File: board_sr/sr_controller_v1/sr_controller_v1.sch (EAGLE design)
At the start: 120 parts, among them IC2 74HC595D, J2 WIRE_HOLE-14AWG, J3 WIRE_HOLE-14AWG, J4 WIRE_HOLE-14AWG, J5 WIRE_HOLE-14AWG, J6 WIRE_HOLE-14AWG, J7 WIRE_HOLE-14AWG, Q1 32kHz, Q3 IRF5210

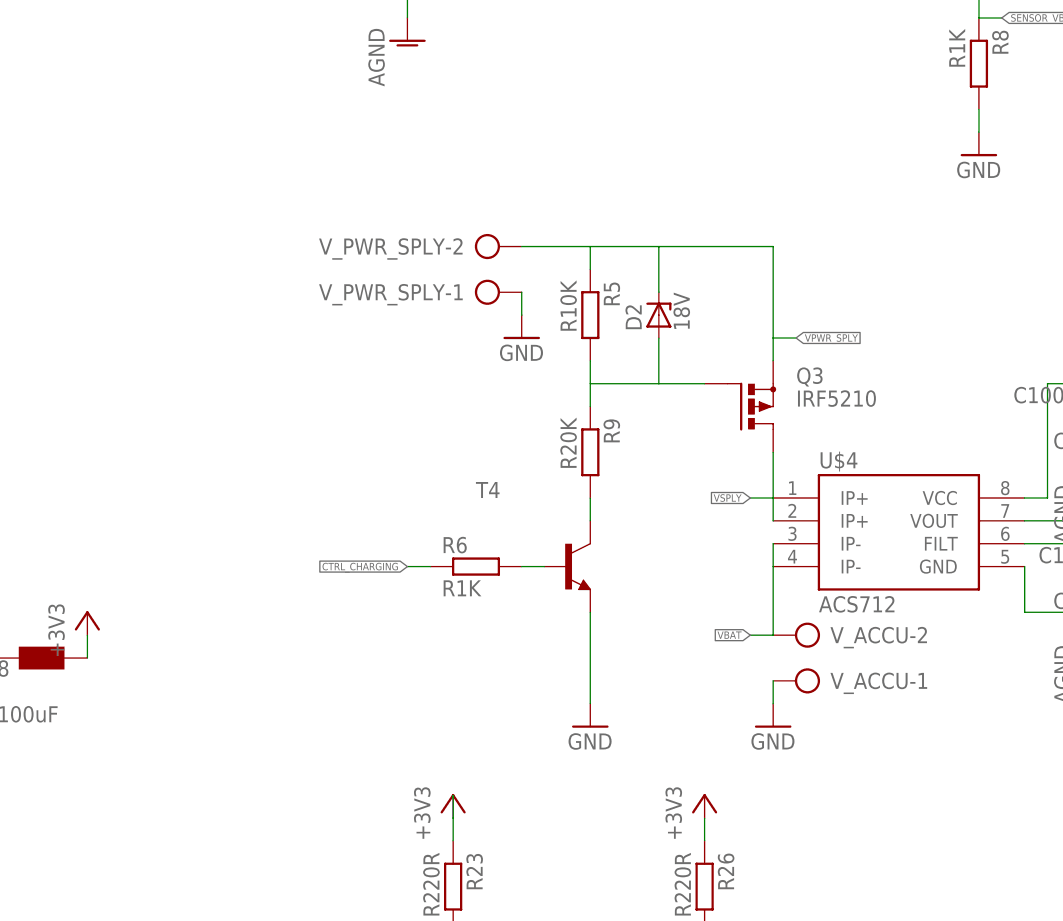
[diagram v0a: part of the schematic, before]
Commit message: Finish Routing PCB ver1 revA
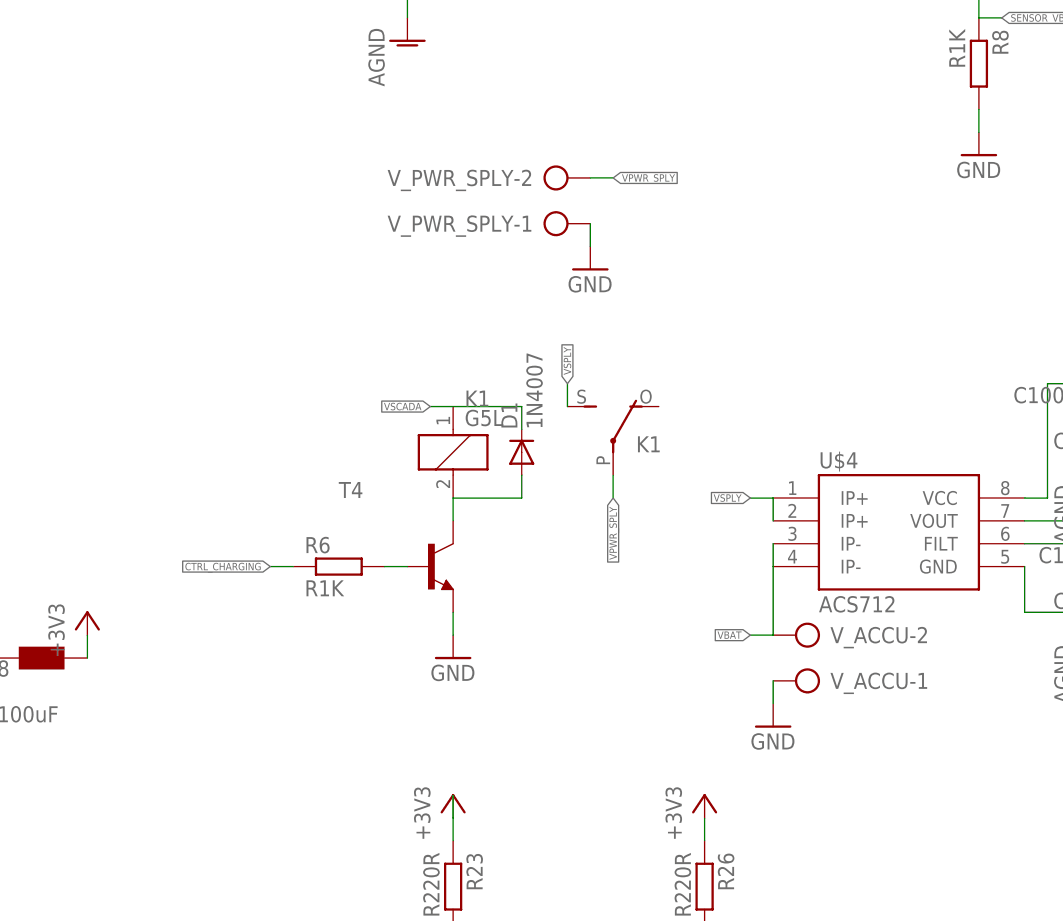
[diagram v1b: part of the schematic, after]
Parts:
- removed D2: 18V, diode:ZENER-DIODEDO41Z10
- removed Q3: IRF5210, transistor-power:PMOSFET_PTO220BV
- removed R5: R10K, resistor:R-EU_R0805
- removed R9: R20K, resistor:R-EU_R0805
- added D1: 1N4007, diode:DIODE-DO214AA
- added K1: G5L, relay:G5L
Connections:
- removed net N$11: D2.A, Q3.G, R5.2, R9.1
- removed net N$14: R9.2, T4.C
- new net N$34: D1.A, K11.2, T4.C
- net VPWR_SPLY: now also K12.P; no longer D2.C, Q3.S, R5.1
- net VSCADA: now also D1.C, K11.1
- net VSPLY: now also K12.S; no longer Q3.D
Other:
- moved on the sheet: R6, T4, V_PWR_SPLY-1, V_PWR_SPLY-2
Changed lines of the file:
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@@
 <part name="V_PWR_SPLY" library="con-ptr500" deviceset="AK300/2" device=""/>
 <part name="V_ACCU" library="con-ptr500" deviceset="AK300/2" device=""/>
-<part name="Q3" library="transistor-power" deviceset="PMOSFET_P" device="TO220BV" value="IRF5210"/>
 <part name="GND15" library="supply1" deviceset="GND" device=""/>
-<part name="R5" library="resistor" deviceset="R-EU_" device="R0805" value="R10K"/>
 <part name="GND16" library="supply1" deviceset="GND" device=""/>
 <part name="GND17" library="supply1" deviceset="GND" device=""/>
@@
 <part name="AGND3" library="supply1" deviceset="AGND" device=""/>
 <part name="GND19" library="supply1" deviceset="GND" device=""/>
-<part name="R9" library="resistor" deviceset="R-EU_" device="R0805" value="R20K"/>
-<part name="D2" library="diode" deviceset="ZENER-DIODE" device="DO41Z10" value="18V"/>
 <part name="U$4" library="SparkFun-AnalogIC" deviceset="ACS712" device=""/>
 <part name="C5" library="resistor" deviceset="C-EU" device="C0805K" value="C100N"/>
@@
 <part name="J6" library="powercube" deviceset="WIRE_HOLE-14AWG" device=""/>
 <part name="J7" library="powercube" deviceset="WIRE_HOLE-14AWG" device=""/>
+<part name="K1" library="relay" deviceset="G5L" device=""/>
+<part name="D1" library="diode" deviceset="DIODE-" device="DO214AA" value="1N4007"/>
 </parts>
 <sheets>
@@
 <instance part="VAC" gate="-1" x="177.8" y="231.14"/>
 <instance part="VAC" gate="-2" x="177.8" y="236.22"/>
-<instance part="V_PWR_SPLY" gate="-1" x="231.14" y="185.42"/>
-<instance part="V_PWR_SPLY" gate="-2" x="231.14" y="190.5"/>
+<instance part="V_PWR_SPLY" gate="-1" x="238.76" y="193.04"/>
+<instance part="V_PWR_SPLY" gate="-2" x="238.76" y="198.12"/>
 <instance part="V_ACCU" gate="-1" x="269.24" y="142.24" rot="R180"/>
 <instance part="V_ACCU" gate="-2" x="269.24" y="147.32" rot="R180"/>
-<instance part="Q3" gate="G$1" x="261.62" y="172.72"/>
 <instance part="GND15" gate="1" x="264.16" y="137.16"/>
-<instance part="R5" gate="G$1" x="243.84" y="182.88" rot="R270"/>
-<instance part="GND16" gate="1" x="236.22" y="180.34"/>
-<instance part="GND17" gate="1" x="243.84" y="137.16"/>
-<instance part="R6" gate="G$1" x="231.14" y="154.94"/>
+<instance part="GND16" gate="1" x="243.84" y="187.96"/>
+<instance part="GND17" gate="1" x="228.6" y="144.78"/>
+<instance part="R6" gate="G$1" x="215.9" y="154.94"/>
 <instance part="R7" gate="G$1" x="287.02" y="223.52" rot="R270"/>
 <instance part="R8" gate="G$1" x="287.02" y="210.82" rot="R270"/>
@@
 <instance part="AGND3" gate="VR1" x="320.04" y="213.36"/>
 <instance part="GND19" gate="1" x="309.88" y="213.36"/>
-<instance part="R9" gate="G$1" x="243.84" y="167.64" rot="R270"/>
-<instance part="D2" gate="G$1" x="251.46" y="182.88" rot="R90"/>
 <instance part="U$4" gate="G$1" x="279.4" y="157.48"/>
 <instance part="C5" gate="G$1" x="299.72" y="170.18" rot="R180"/>
@@
 <instance part="U$6" gate="G$1" x="48.26" y="78.74"/>
 <instance part="U$7" gate="G$1" x="48.26" y="45.72"/>
-<instance part="T4" gate="G$1" x="241.3" y="154.94"/>
+<instance part="T4" gate="G$1" x="226.06" y="154.94"/>
 <instance part="U$8" gate="G$1" x="347.98" y="106.68"/>
 <instance part="GND45" gate="1" x="335.28" y="93.98"/>
@@
 <instance part="J6" gate="G$1" x="398.78" y="160.02"/>
 <instance part="J7" gate="G$1" x="398.78" y="149.86"/>
+<instance part="K1" gate="1" x="228.6" y="167.64"/>
+<instance part="K1" gate="2" x="246.38" y="167.64"/>
+<instance part="D1" gate="G$1" x="236.22" y="167.64" rot="R90"/>
 </instances>
 <busses>
@@
 </segment>
 <segment>
-<wire x1="243.84" y1="149.86" x2="243.84" y2="139.7" width="0.1524" layer="91"/>
+<wire x1="228.6" y1="149.86" x2="228.6" y2="147.32" width="0.1524" layer="91"/>
 <pinref part="GND17" gate="1" pin="GND"/>
 <pinref part="T4" gate="G$1" pin="E"/>
@@
 <pinref part="GND16" gate="1" pin="GND"/>
 <pinref part="V_PWR_SPLY" gate="-1" pin="KL"/>
-<wire x1="236.22" y1="182.88" x2="236.22" y2="185.42" width="0.1524" layer="91"/>
+<wire x1="243.84" y1="190.5" x2="243.84" y2="193.04" width="0.1524" layer="91"/>
 </segment>
 <segment>
@@
 </segment>
 </net>
-<net name="N$11" class="0">
-<segment>
-<pinref part="Q3" gate="G$1" pin="G"/>
-<pinref part="R5" gate="G$1" pin="2"/>
-<wire x1="243.84" y1="177.8" x2="243.84" y2="175.26" width="0.1524" layer="91"/>
-<wire x1="256.54" y1="175.26" x2="251.46" y2="175.26" width="0.1524" layer="91"/>
-<pinref part="D2" gate="G$1" pin="A"/>
-<wire x1="251.46" y1="175.26" x2="243.84" y2="175.26" width="0.1524" layer="91"/>
-<wire x1="251.46" y1="180.34" x2="251.46" y2="175.26" width="0.1524" layer="91"/>
-<pinref part="R9" gate="G$1" pin="1"/>
-<wire x1="243.84" y1="172.72" x2="243.84" y2="175.26" width="0.1524" layer="91"/>
-</segment>
-</net>
 <net name="VPWR_SPLY" class="0">
 <segment>
-<pinref part="Q3" gate="G$1" pin="S"/>
-<wire x1="243.84" y1="190.5" x2="251.46" y2="190.5" width="0.1524" layer="91"/>
-<wire x1="251.46" y1="190.5" x2="264.16" y2="190.5" width="0.1524" layer="91"/>
-<wire x1="264.16" y1="190.5" x2="264.16" y2="180.34" width="0.1524" layer="91"/>
-<pinref part="R5" gate="G$1" pin="1"/>
-<wire x1="264.16" y1="180.34" x2="264.16" y2="177.8" width="0.1524" layer="91"/>
-<wire x1="243.84" y1="187.96" x2="243.84" y2="190.5" width="0.1524" layer="91"/>
-<pinref part="D2" gate="G$1" pin="C"/>
-<wire x1="251.46" y1="185.42" x2="251.46" y2="190.5" width="0.1524" layer="91"/>
 <pinref part="V_PWR_SPLY" gate="-2" pin="KL"/>
-<wire x1="236.22" y1="190.5" x2="243.84" y2="190.5" width="0.1524" layer="91"/>
-<label x="266.7" y="180.34" size="0.8128" layer="95" xref="yes"/>
-<wire x1="266.7" y1="180.34" x2="264.16" y2="180.34" width="0.1524" layer="91"/>
+<wire x1="243.84" y1="198.12" x2="246.38" y2="198.12" width="0.1524" layer="91"/>
+<label x="246.38" y="198.12" size="0.8128" layer="95" xref="yes"/>
+</segment>
+<segment>
+<pinref part="K1" gate="2" pin="P"/>
+<wire x1="246.38" y1="165.1" x2="246.38" y2="162.56" width="0.1524" layer="91"/>
+<label x="246.38" y="162.56" size="0.8128" layer="95" rot="R270" xref="yes"/>
 </segment>
 </net>
@@
 <segment>
 <pinref part="R6" gate="G$1" pin="2"/>
-<wire x1="238.76" y1="154.94" x2="236.22" y2="154.94" width="0.1524" layer="91"/>
+<wire x1="223.52" y1="154.94" x2="220.98" y2="154.94" width="0.1524" layer="91"/>
 <pinref part="T4" gate="G$1" pin="B"/>
 </segment>
@@
 <segment>
 <pinref part="R6" gate="G$1" pin="1"/>
-<wire x1="226.06" y1="154.94" x2="223.52" y2="154.94" width="0.1524" layer="91"/>
-<label x="223.52" y="154.94" size="0.8128" layer="95" rot="R180" xref="yes"/>
+<wire x1="210.82" y1="154.94" x2="208.28" y2="154.94" width="0.1524" layer="91"/>
+<label x="208.28" y="154.94" size="0.8128" layer="95" rot="R180" xref="yes"/>
 </segment>
 <segment>
@@
 </segment>
 </net>
-<net name="N$14" class="0">
-<segment>
-<pinref part="R9" gate="G$1" pin="2"/>
-<wire x1="243.84" y1="160.02" x2="243.84" y2="162.56" width="0.1524" layer="91"/>
-<pinref part="T4" gate="G$1" pin="C"/>
-</segment>
-</net>
 <net name="VSPLY" class="0">
 <segment>
-<pinref part="Q3" gate="G$1" pin="D"/>
 <pinref part="U$4" gate="G$1" pin="IP+@1"/>
-<wire x1="264.16" y1="167.64" x2="264.16" y2="162.56" width="0.1524" layer="91"/>
 <pinref part="U$4" gate="G$1" pin="IP+@2"/>
 <wire x1="264.16" y1="162.56" x2="264.16" y2="160.02" width="0.1524" layer="91"/>
@@
 <wire x1="332.74" y1="228.6" x2="330.2" y2="228.6" width="0.1524" layer="91"/>
 <label x="330.2" y="228.6" size="0.8128" layer="95" rot="R180" xref="yes"/>
+</segment>
+<segment>
+<pinref part="K1" gate="2" pin="S"/>
+<wire x1="241.3" y1="172.72" x2="241.3" y2="175.26" width="0.1524" layer="91"/>
+<label x="241.3" y="175.26" size="0.8128" layer="95" rot="R90" xref="yes"/>
 </segment>
 </net>
@@
 <label x="403.86" y="149.86" size="0.8128" layer="95" xref="yes"/>
 </segment>
+<segment>
+<pinref part="K1" gate="1" pin="1"/>
+<pinref part="D1" gate="G$1" pin="C"/>
+<wire x1="228.6" y1="172.72" x2="236.22" y2="172.72" width="0.1524" layer="91"/>
+<wire x1="236.22" y1="172.72" x2="236.22" y2="170.18" width="0.1524" layer="91"/>
+<wire x1="228.6" y1="172.72" x2="226.06" y2="172.72" width="0.1524" layer="91"/>
+<label x="226.06" y="172.72" size="0.8128" layer="95" rot="R180" xref="yes"/>
+</segment>
 </net>
 <net name="VSCPC" class="0">
@@
 </segment>
 </net>
+<net name="N$34" class="0">
+<segment>
+<pinref part="K1" gate="1" pin="2"/>
+<pinref part="D1" gate="G$1" pin="A"/>
+<wire x1="228.6" y1="162.56" x2="236.22" y2="162.56" width="0.1524" layer="91"/>
+<wire x1="236.22" y1="162.56" x2="236.22" y2="165.1" width="0.1524" layer="91"/>
+<pinref part="T4" gate="G$1" pin="C"/>
+<wire x1="228.6" y1="162.56" x2="228.6" y2="160.02" width="0.1524" layer="91"/>
+</segment>
+</net>
